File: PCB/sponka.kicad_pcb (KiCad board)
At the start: 2 copper layers, 87.1 x 13.3 mm, 31 parts, among them J1 Conn_01x03_Pin, J2 USB_C_Receptacle_USB2.0_14P, J3 Conn_01x02_Socket, J4 Conn_01x05_Pin, SW1 SW_Push, SW2 SW_SPDT, U1 CH32V003FxUx, U2 TP4057, U3 AP2127K-3.3

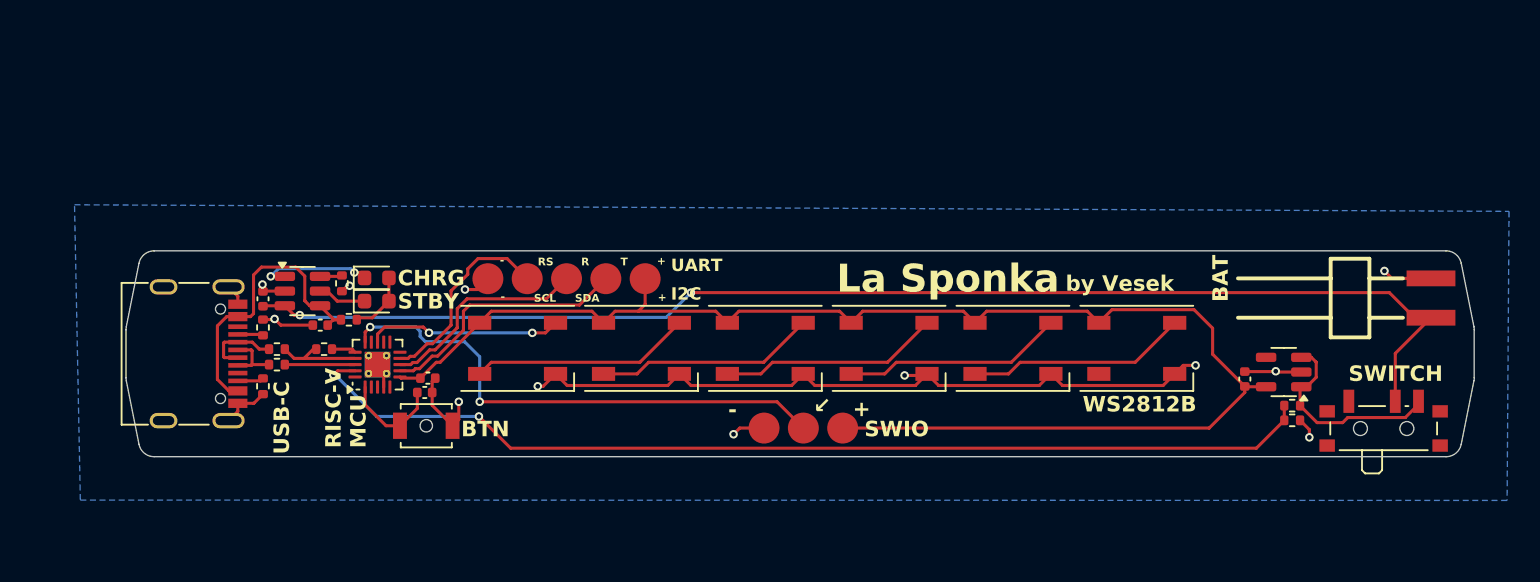
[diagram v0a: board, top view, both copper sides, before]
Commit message: Made smol :) Anyway, this is just WIP, still working on it
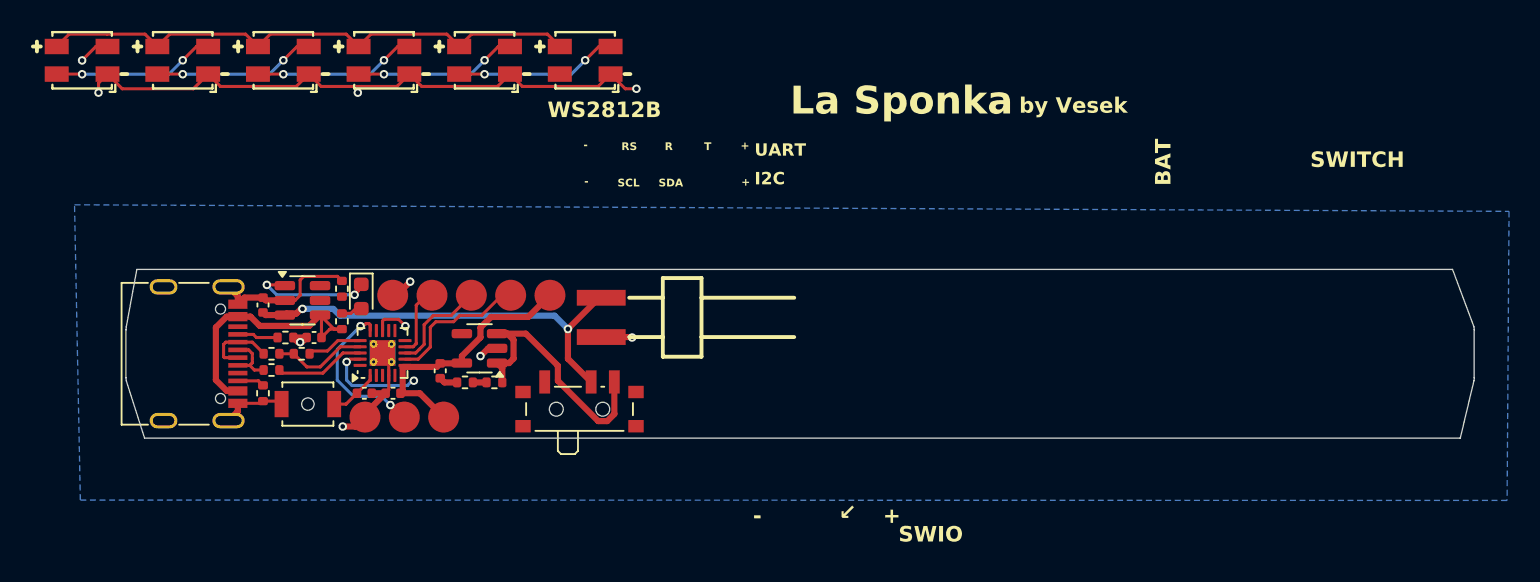
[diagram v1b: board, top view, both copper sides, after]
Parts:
- removed D1, D2, D3, D4, D5, D6: WS2812B, LED_SMD:LED_WS2812B_PLCC4_5.0x5.0mm_P3.2mm
- removed D_STDBY1: LED, LED_SMD:LED_0603_1608Metric
- added LED1: WS2812B-MINI, sponka:LED-SMD_4P-L3.5-W3.5-TL_WS2812B, F.Cu at (97.9, 82.4)
- added LED2: WS2812B-MINI, sponka:LED-SMD_4P-L3.5-W3.5-TL_WS2812B, F.Cu at (104.4, 82.4)
- added LED3: WS2812B-MINI, sponka:LED-SMD_4P-L3.5-W3.5-TL_WS2812B, F.Cu at (110.9, 82.4)
- added LED4: WS2812B-MINI, sponka:LED-SMD_4P-L3.5-W3.5-TL_WS2812B, F.Cu at (117.4, 82.4)
- added LED5: WS2812B-MINI, sponka:LED-SMD_4P-L3.5-W3.5-TL_WS2812B, F.Cu at (123.9, 82.4)
- added LED6: WS2812B-MINI, sponka:LED-SMD_4P-L3.5-W3.5-TL_WS2812B, F.Cu at (130.4, 82.4)
- moved J3 53.6 mm to (131.4, 99.0), turned to 90 degrees
- moved R8 53.5 mm to (122.6, 103.2), turned to 180 degrees
- moved C5 52.0 mm to (121.0, 102.5), turned to -90 degrees
- moved U3 52.0 mm to (123.5, 101.0)
- moved SW2 52.0 mm to (130.0, 104.6)
- moved R7 51.6 mm to (124.5, 103.2)
- moved J1 25.8 mm to (118.7, 105.4)
- moved SW1 7.78 mm to (112.5, 104.6), turned to 180 degrees
- moved J4 6.24 mm to (123.0, 97.6)
- moved C2 3.90 mm to (116.1, 103.9)
- moved C1 2.45 mm to (118.0, 103.9), turned to 180 degrees
- moved R1 1.59 mm to (111.0, 100.3), turned to 180 degrees
- moved D_CHRG1 1.56 mm to (115.9, 97.7), turned to -90 degrees
- moved R9 1.48 mm to (112.0, 101.3)
- moved C3 0.89 mm to (112.8, 100.3)
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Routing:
- net /Power management/BATT_DIV: track 66.8 -> 7.62 mm
- net Net-(J3-Pin_2): track 83.5 -> 27.5 mm
- net +3V3: track 93.7 -> 53.0 mm
- net Net-(J1-Pin_2): track 33.7 -> 11.2 mm
- net Net-(D1-DOUT): track 14.3 -> 0.00 mm
- net Net-(D5-DOUT): track 14.3 -> 0.00 mm
- net Net-(D4-DOUT): track 14.3 -> 0.00 mm
- net Net-(D3-DOUT): track 14.3 -> 0.00 mm
- net Net-(D2-DOUT): track 14.3 -> 0.00 mm
- net Net-(LED5-DOUT): track 0.00 -> 10.5 mm, vias 0 -> 2
- net Net-(LED3-DOUT): track 0.00 -> 10.5 mm, vias 0 -> 2
- net Net-(LED2-DOUT): track 0.00 -> 10.5 mm, vias 0 -> 2
- net Net-(LED1-DOUT): track 0.00 -> 10.5 mm, vias 0 -> 2
- net Net-(LED4-DOUT): track 0.00 -> 10.5 mm, vias 0 -> 2
- net /LED Row/Row_DIN: track 12.8 -> 4.37 mm
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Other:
- board size 87.1 x 13.3 mm -> 87.1 x 10.9 mm
- board text removed: "BTN"
- board text removed: "CHRG"
- board text removed: "RISC-V MCU"
- board text removed: "STBY"
- board text removed: "USB-C"

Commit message: Progress update
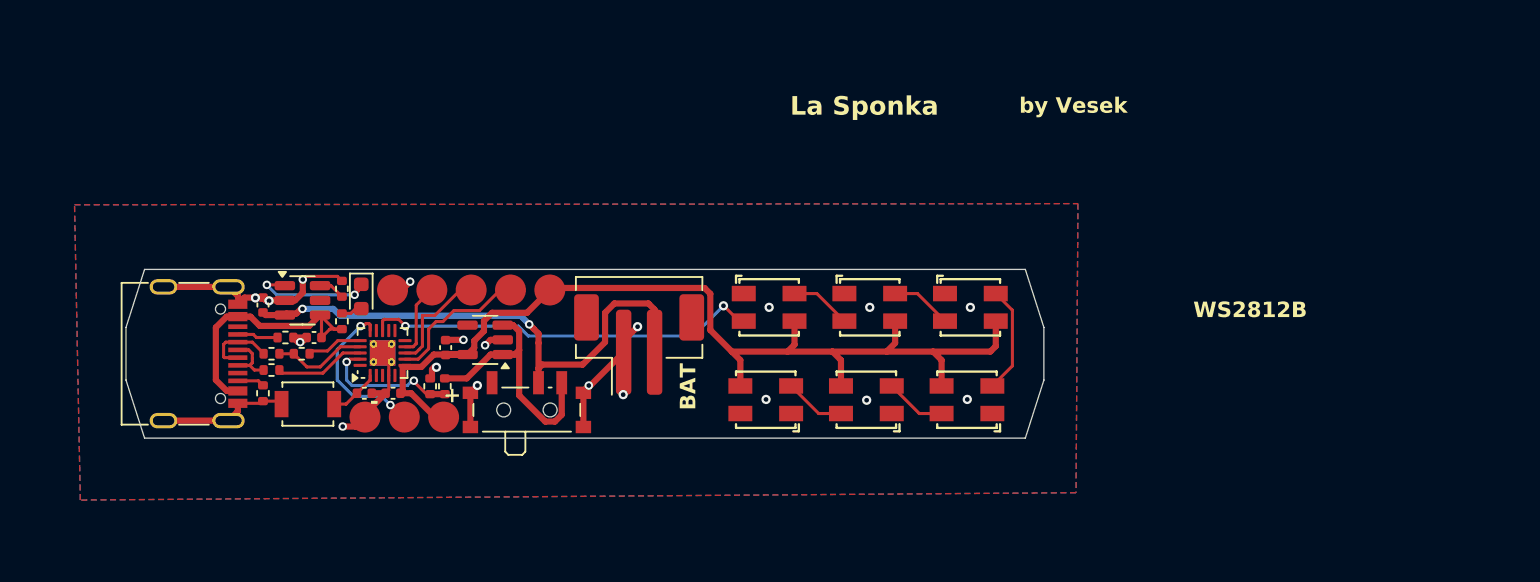
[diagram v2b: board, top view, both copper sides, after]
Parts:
- J3: footprint sponka:HDR-SMD_2P-P2.54-H-M-W13.3-N -> Connector_JST:JST_PH_B2B-PH-SM4-TB_1x02-1MP_P2.00mm_Vertical
- SW1: footprint Button_Switch_SMD:SW_SPST_B3U-1000P-B -> Button_Switch_SMD:SW_SPST_B3U-1000P
- moved LED1 47.2 mm to (142.2, 98.3), turned to 180 degrees
- moved LED2 47.2 mm to (148.8, 98.3), turned to 180 degrees
- moved LED3 47.2 mm to (155.2, 98.3), turned to 180 degrees
- moved LED4 43.6 mm to (155.0, 104.3)
- moved LED5 33.0 mm to (148.5, 104.3)
- moved LED6 24.8 mm to (142.0, 104.3)
- moved SW2 3.40 mm to (126.6, 104.7)
- moved R7 3.21 mm to (121.3, 103.5), turned to -90 degrees
- moved J3 3.01 mm to (133.8, 100.8), turned to 0 degrees
- moved R8 2.26 mm to (120.3, 103.5), turned to 90 degrees
- moved C5 1.54 mm to (121.3, 101.0), turned to 90 degrees
- moved U3 0.66 mm to (123.9, 100.5)
- moved J4 0.34 mm to (123.0, 97.2)
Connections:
- SW2 pad : (no net) -> GND
- U2 pad 5: Net-(D_STDBY1-K) -> unconnected-(U2-STDBY-Pad5)
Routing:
- net GND: track 69.4 -> 47.6 mm, vias 8 -> 19
- net /LED Row/Row_DIN: track 4.37 -> 25.7 mm
- net +3V3: track 53.0 -> 64.2 mm
- net Net-(J3-Pin_2): track 27.5 -> 35.1 mm
- net Net-(LED5-DOUT): track 10.5 -> 3.96 mm, vias 2 -> 0
- net Net-(LED4-DOUT): track 10.5 -> 3.96 mm, vias 2 -> 0
- net Net-(LED2-DOUT): track 10.5 -> 3.96 mm, vias 2 -> 0
- net Net-(LED1-DOUT): track 10.5 -> 3.96 mm, vias 2 -> 0
- net Net-(LED3-DOUT): track 10.5 -> 6.95 mm, vias 2 -> 0
- net Net-(U2-PROG): track 0.00 -> 1.71 mm
- net /Power management/BATT_DIV: track 7.62 -> 9.13 mm
- net Net-(SW2-C): track 17.8 -> 16.6 mm
- net /RX/SDA: track 6.58 -> 7.13 mm
- added copper zone on F.Cu, net GND
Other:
- board size 87.1 x 10.9 mm -> 59.3 x 10.9 mm
- board text added: "D"
- board text added: "RTS"
- board text added: "RX"
- board text added: "TX"
- board text removed: "R"
- board text removed: "RS"
- board text removed: "SWITCH"
- board text removed: "T"
